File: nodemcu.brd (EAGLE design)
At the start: 50.5 x 49.5 mm, 6 parts

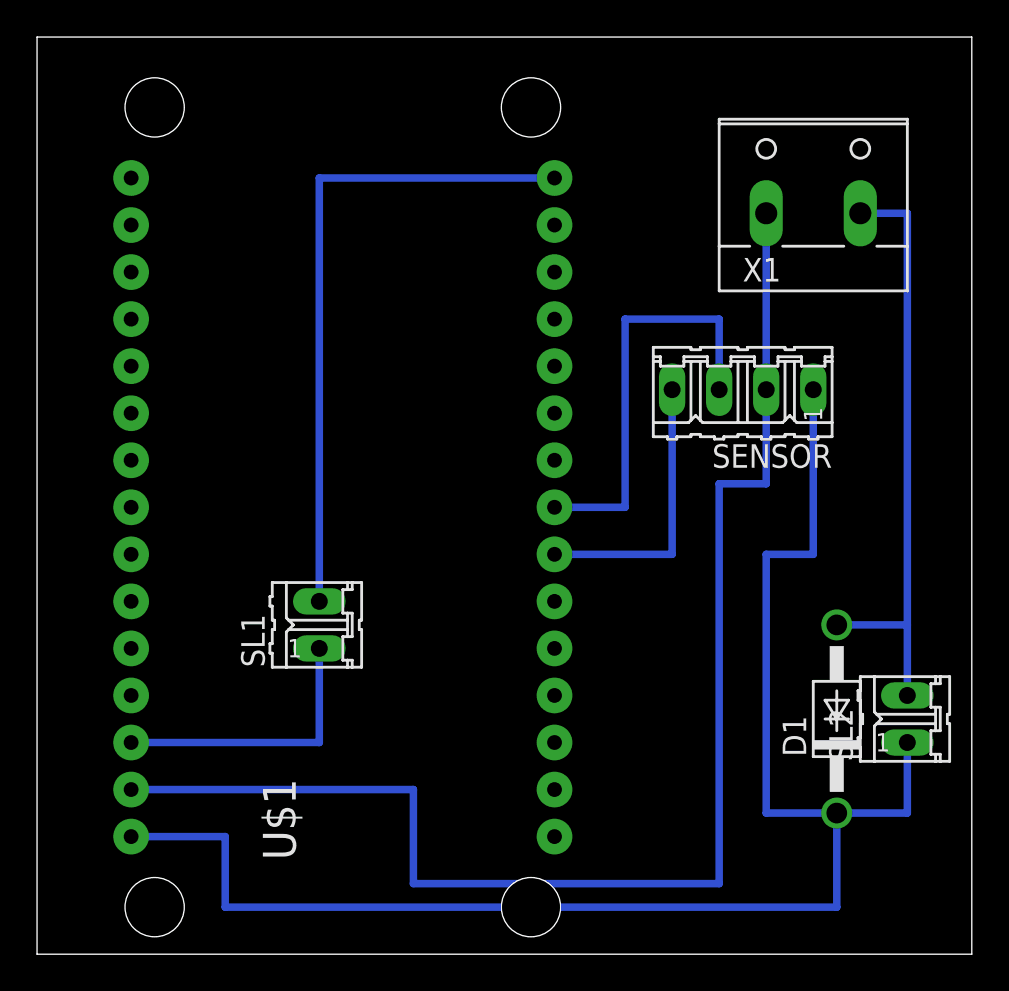
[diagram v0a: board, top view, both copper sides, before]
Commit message: uprava desky
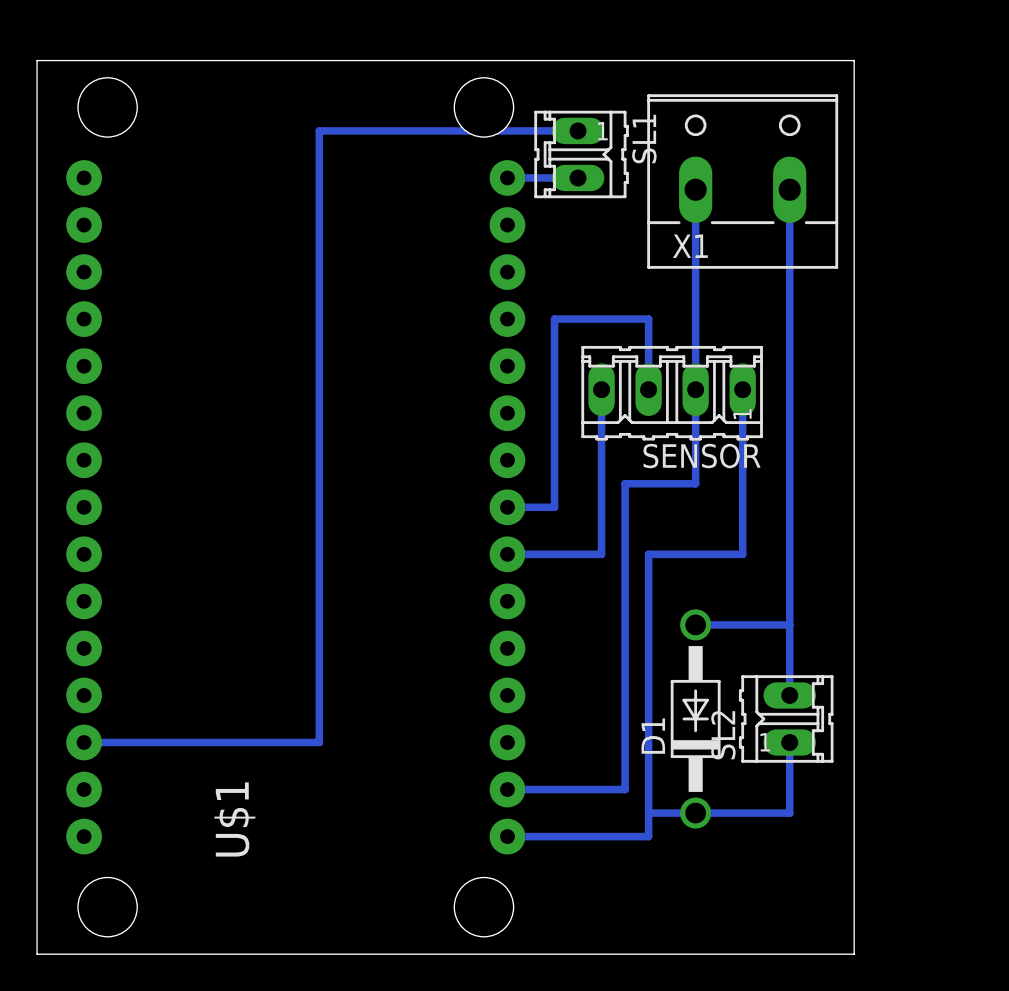
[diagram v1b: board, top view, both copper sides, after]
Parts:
- moved SL1 29.0 mm to (29.2, 43.2), turned to 270 degrees
- moved D1 7.62 mm to (35.6, 12.7)
- moved SL2 6.35 mm to (40.6, 12.7)
- moved X1 4.02 mm to (38.1, 41.9)
- moved SENSOR 3.81 mm to (34.3, 30.5)
- moved U$1 2.54 mm to (14.0, 24.1)
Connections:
- new net N$6: U$1.VIN
- net +3V3: now also U$1.3V3@2; no longer U$1.VIN
- net GND: now also U$1.GND@3; no longer U$1.GND@1
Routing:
- net N$4: track 15.2 -> 59.7 mm
- net +3V3: track 83.8 -> 48.3 mm
- net GND: track 75.6 -> 42.5 mm
- net N$1: track 35.6 -> 3.81 mm
- net N$2: track 15.2 -> 14.0 mm
- net N$3: track 22.9 -> 21.6 mm
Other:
- board size 50.5 x 49.5 mm -> 44.1 x 48.2 mm
